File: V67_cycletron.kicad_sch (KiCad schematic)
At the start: 49 parts, among them J1 USB_C_Receptacle_USB2.0_16P, J10 Screw_Terminal_01x02, J11 PINHD_1x2_Male, J13 PINHD_2x2_Male, J2 PINHD_1x2_Male, J3 PINHD_1x2_Male, J4 PINHD_1x4_Male, J5 PINHD_1x4_Male, J6 PINHD_1x4_Male, J7 PINHD_1x4_Male, J8 PINHD_2x4_Male, J9 PINHD_1x3_Male, Q1 IRF1324, U2 LM1117DT-3.3, U3 L7805, U4 ESP32-S3-WROOM-1

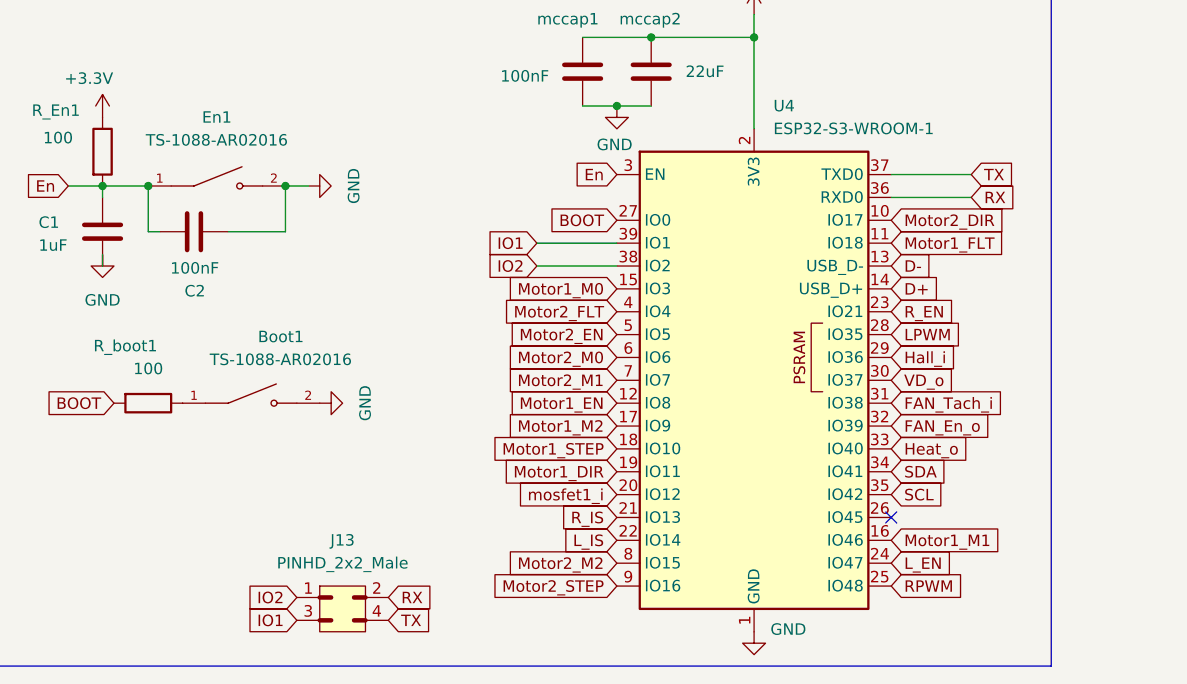
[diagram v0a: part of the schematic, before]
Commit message: changes to pin placement
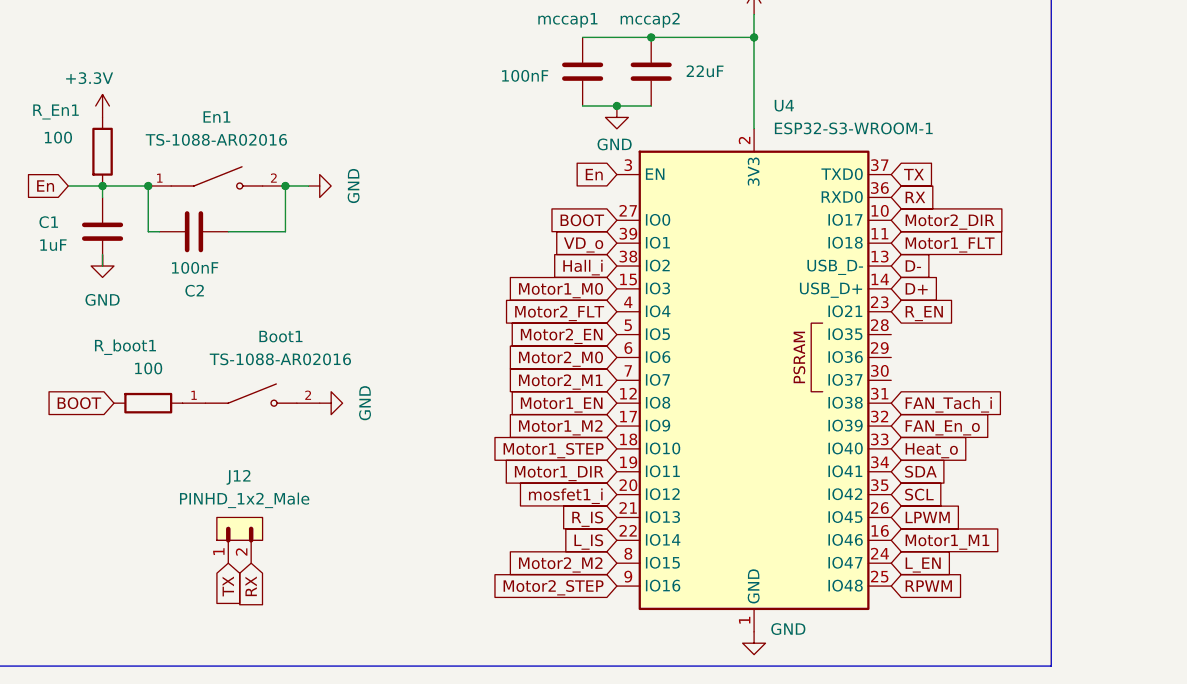
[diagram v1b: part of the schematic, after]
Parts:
- removed J13: PINHD_2x2_Male, Connector_PinHeader_2.54mm:PinHeader_2x02_P2.54mm_Vertical, symbol PCM_SL_Pin_Headers:PINHD_2x2_Male
- added J12: PINHD_1x2_Male, Connector_PinHeader_2.54mm:PinHeader_1x02_P2.54mm_Vertical, symbol PCM_SL_Pin_Headers:PINHD_1x2_Male
- J11, J2, J3: LCSC (none) -> C5360898
- J4, J5, J6, J7: LCSC (none) -> C5116483
- J8: LCSC (none) -> C5156679
- J9: LCSC (none) -> C5360899
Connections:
- net IO1 is gone; now on net Therm-: U4.39 (IO1)
- net IO2 is gone; now on net Hall_i: U4.38 (IO2)
- net Hall_i: no longer U4.29 (IO36)
- net LPWM: now also U4.26 (IO45); no longer U4.28 (IO35)
- net RX: now also J12.2
- net TX: now also J12.1
- net Therm-: no longer U4.30 (IO37)
- no-connect marks 3 -> 2
